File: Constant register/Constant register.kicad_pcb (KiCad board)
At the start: 2 copper layers, 76.2 x 38.1 mm, 30 parts, among them J1 Conn_01x16, J2 Conn_01x04, U1 74HCT574, U2 74HCT541

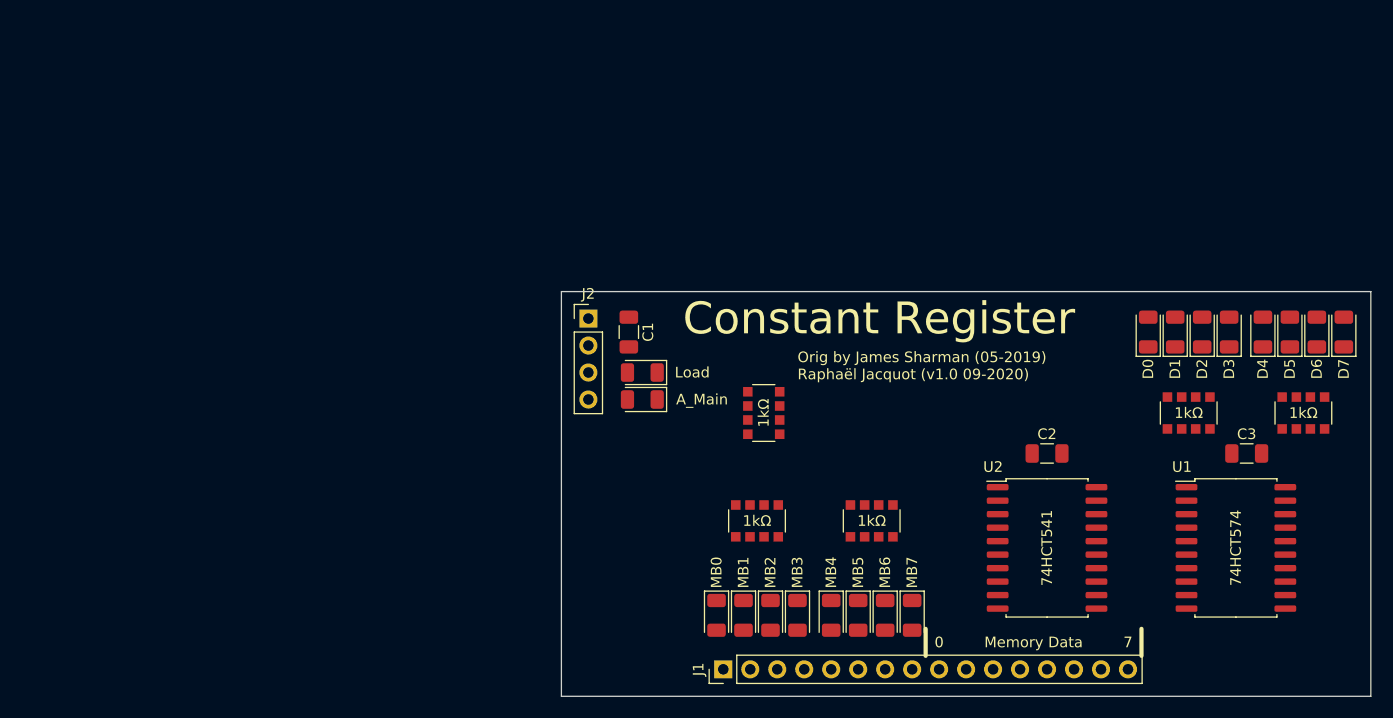
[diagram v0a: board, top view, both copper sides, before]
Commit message: move to Constant Register v2.0
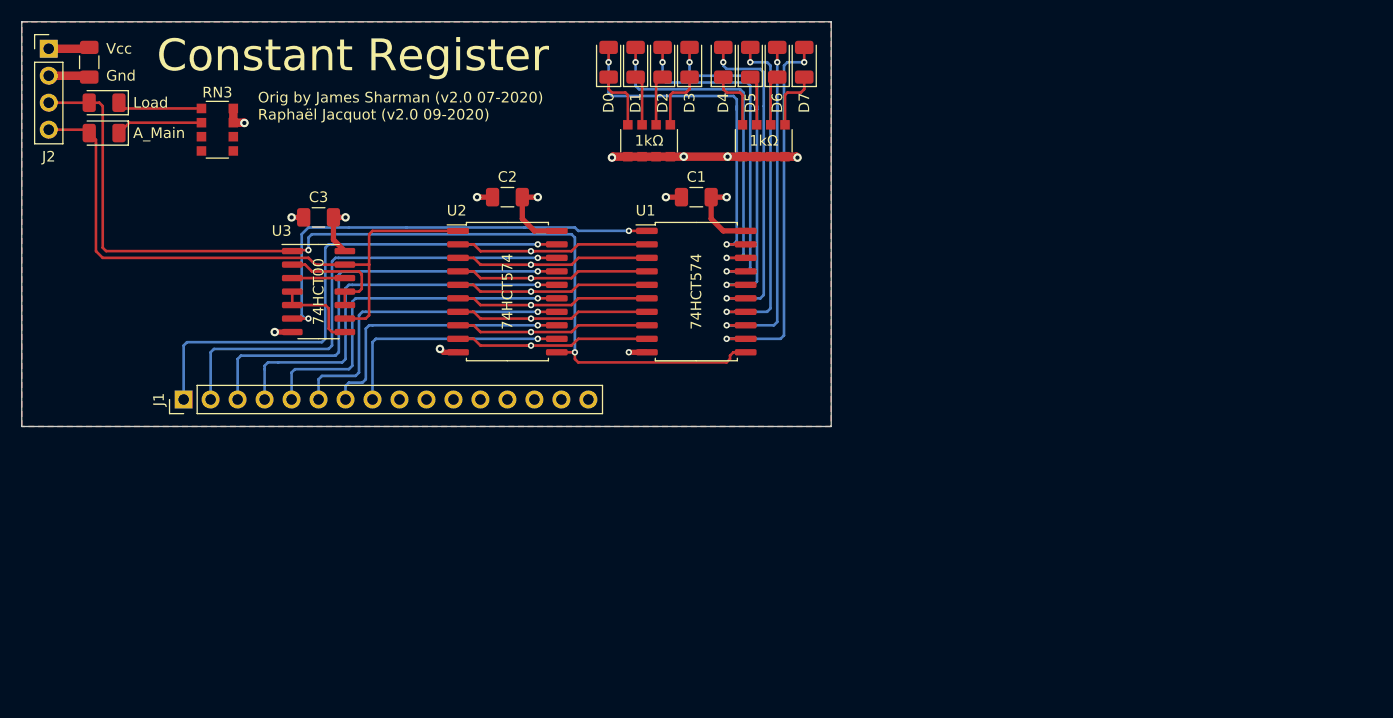
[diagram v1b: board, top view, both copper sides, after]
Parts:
- removed D11: MB0, LED_SMD:LED_1206_3216Metric
- removed D12: MB1, LED_SMD:LED_1206_3216Metric
- removed D13: MB2, LED_SMD:LED_1206_3216Metric
- removed D14: MB3, LED_SMD:LED_1206_3216Metric
- removed D15: MB4, LED_SMD:LED_1206_3216Metric
- removed D16: MB5, LED_SMD:LED_1206_3216Metric
- removed D17: MB6, LED_SMD:LED_1206_3216Metric
- removed D18: MB7, LED_SMD:LED_1206_3216Metric
- removed RN4, RN5: R_Pack04, Resistor_SMD:R_Array_Convex_4x1206
- added C4: C, Capacitor_SMD:C_1206_3216Metric, F.Cu at (82.5, 67.3)
- added U3: 74HCT00, Package_SO:SOIC-14_3.9x8.7mm_P1.27mm, F.Cu at (104.1, 88.9)
- U2: value 74HCT541 -> 74HCT574
- moved C3 90.2 mm to (104.1, 81.9), turned to 180 degrees
- moved RN3 57.9 mm to (94.6, 73.7)
- moved RN1 56.9 mm to (135.3, 74.7)
- moved RN2 56.9 mm to (146.1, 74.7)
- moved D1 56.8 mm to (131.4, 67.3)
- moved D4 56.8 mm to (139.1, 67.3)
- moved D6 56.8 mm to (144.8, 67.3)
- moved D7 56.8 mm to (147.3, 67.3)
- moved J1 56.8 mm to (91.4, 99.1)
- moved J2 56.8 mm to (78.7, 66.0)
- moved D2 56.8 mm to (134.0, 67.3)
- moved D3 56.8 mm to (136.5, 67.3)
- moved D5 56.8 mm to (142.2, 67.3)
- moved D8 56.8 mm to (149.9, 67.3)
- moved D9 56.7 mm to (83.9, 71.1)
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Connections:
- U1 pad 1: GND -> /Reg_Valid
- U2 pad 11: /MB7 -> /Load
- U2 pad 12: /MB6 -> /MB7
- U2 pad 13: /MB5 -> /MB6
- U2 pad 14: /MB4 -> /MB5
- U2 pad 15: /MB3 -> /MB4
- U2 pad 16: /MB2 -> /MB3
- U2 pad 17: /MB1 -> /MB2
- U2 pad 18: /MB0 -> /MB1
- U2 pad 19: GND -> /MB0
- U2 pad 2: /Reg0 -> /MD0
- U2 pad 3: /Reg1 -> /MD1
- U2 pad 4: /Reg2 -> /MD2
- U2 pad 5: /Reg3 -> /MD3
- U2 pad 6: /Reg4 -> /MD4
- U2 pad 7: /Reg5 -> /MD5
- U2 pad 8: /Reg6 -> /MD6
- U2 pad 9: /Reg7 -> /MD7
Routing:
- net /Load: track 0.00 -> 94.5 mm, vias 0 -> 2
- net /A_Main: track 0.00 -> 60.1 mm
- net /MB0: track 0.00 -> 49.2 mm, vias 0 -> 1
- net /MB1: track 0.00 -> 45.4 mm, vias 0 -> 1
- net /MD0: track 0.00 -> 44.1 mm, vias 0 -> 1
- net /Reg_Valid: track 0.00 -> 42.8 mm, vias 0 -> 2
- net /MB2: track 0.00 -> 41.6 mm, vias 0 -> 1
- net /MD1: track 0.00 -> 40.3 mm, vias 0 -> 1
- net /MB3: track 0.00 -> 37.7 mm, vias 0 -> 1
- net /MD2: track 0.00 -> 36.5 mm, vias 0 -> 1
- net /Reg7: track 0.00 -> 36.2 mm, vias 0 -> 2
- net /MB4: track 0.00 -> 33.9 mm, vias 0 -> 1
- net /Reg0: track 0.00 -> 33.1 mm, vias 0 -> 2
- net /Reg3: track 0.00 -> 33.1 mm, vias 0 -> 2
- net /Reg6: track 0.00 -> 32.9 mm, vias 0 -> 2
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- added copper zone on B.Cu, net GND
- added copper zone on F.Cu, net GND
- added copper zone on In2.Cu, net GND
- added copper zone on In1.Cu, net VCC
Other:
- copper layers 2 -> 4
- board text added: "Gnd"
- board text added: "Orig by James Sharman (v2.0 07-2020) Raphaël Jacquot (v2.0 09-2020)"
- board text added: "Vcc"
- board text removed: "0"
- board text removed: "7"
- board text removed: "Memory Data"
- board text removed: "Orig by James Sharman (05-2019) Raphaël Jacquot (v1.0 09-2020)"
